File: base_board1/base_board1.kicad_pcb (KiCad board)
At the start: 4 copper layers, 99.4 x 100 mm, 161 parts, among them J1 DF40C-60DS-0.4V_51_, J2 DF40C-60DS-0.4V_51_, J3 Conn_01x30, J4 Conn_01x30, J5 Conn_01x30, J6 Conn_01x30

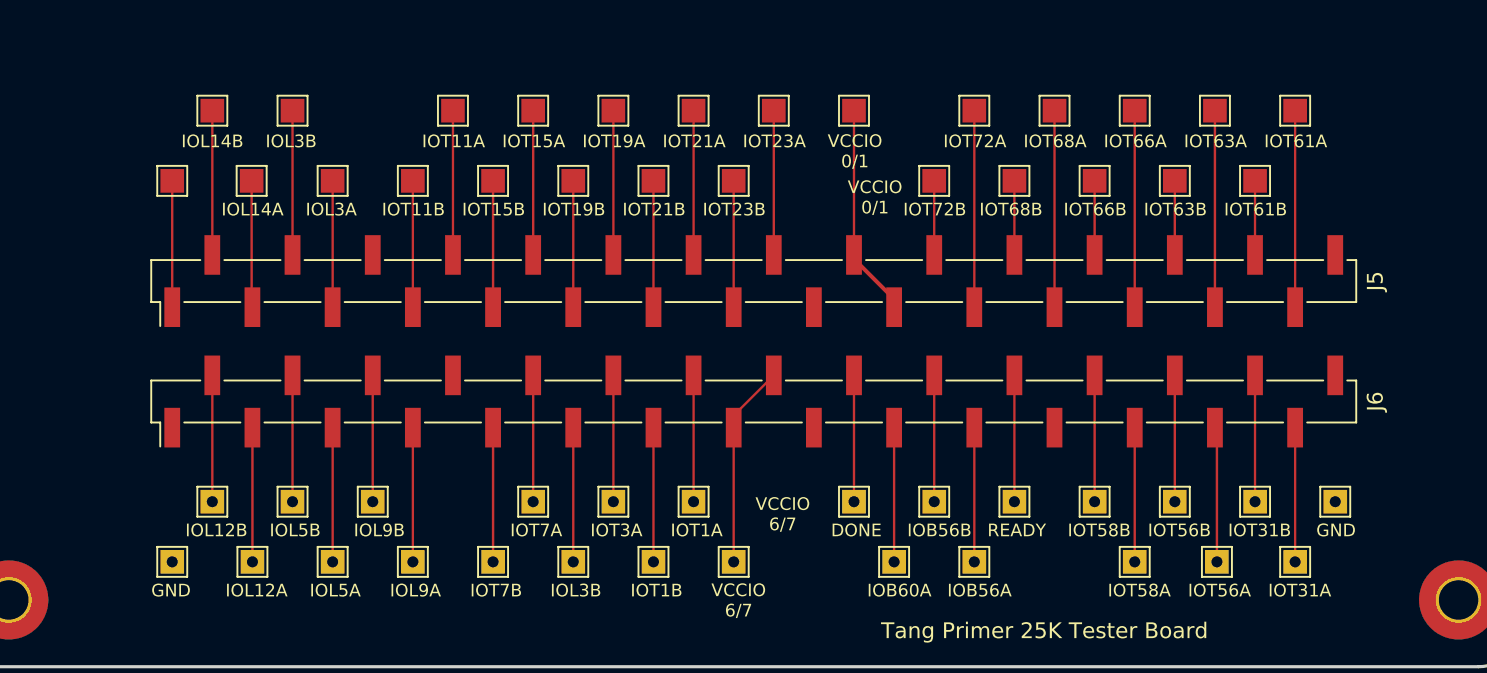
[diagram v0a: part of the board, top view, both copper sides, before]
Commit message: 1219
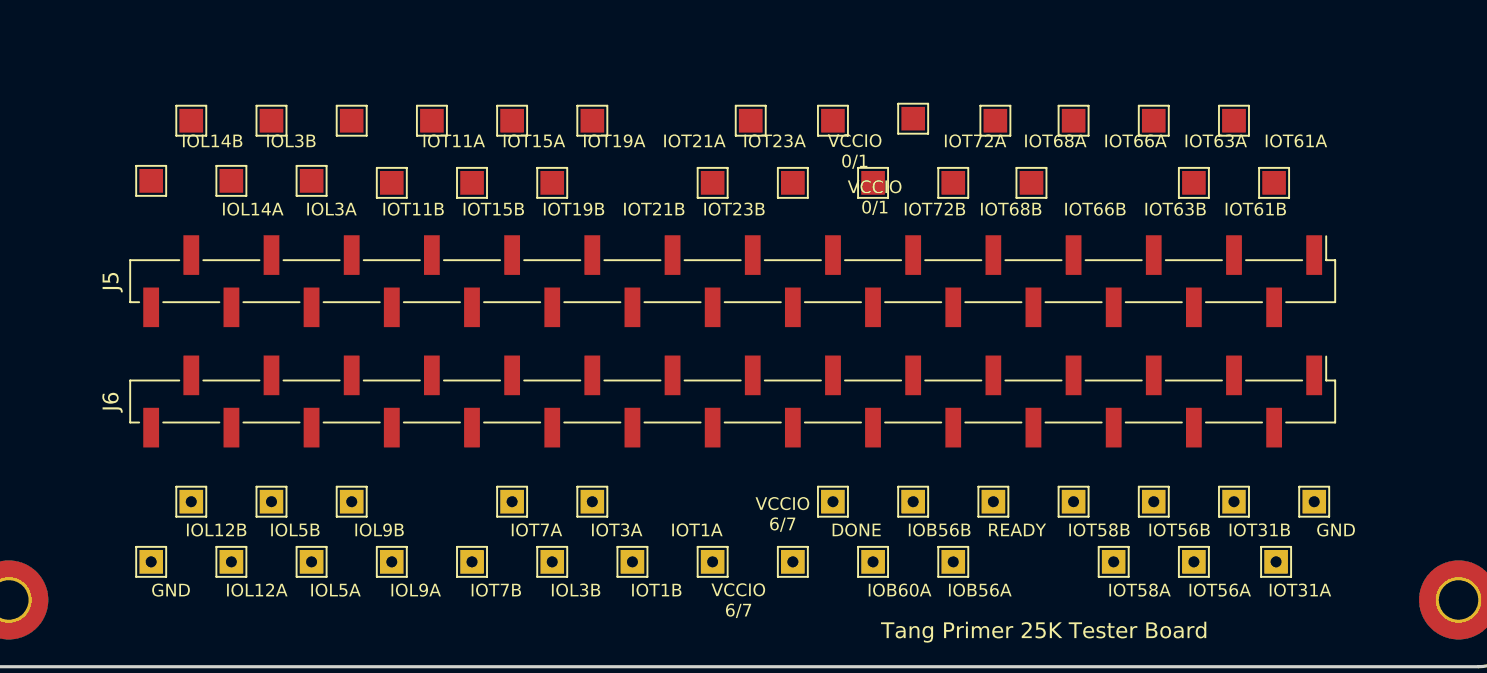
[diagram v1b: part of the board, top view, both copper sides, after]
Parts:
- moved TP69 70.0 mm to (137.3, 146.7)
- moved TP70 69.9 mm to (137.3, 122.6)
- moved TP123 67.5 mm to (206.0, 150.5)
- moved TP124 67.4 mm to (205.9, 126.5)
- moved TP71 64.9 mm to (139.8, 150.5)
- moved TP72 64.8 mm to (139.8, 126.4)
- moved TP122 62.3 mm to (203.3, 122.6)
- moved TP121 62.3 mm to (203.3, 146.7)
- moved TP73 60.0 mm to (142.4, 146.7)
- moved TP74 59.8 mm to (142.4, 122.6)
- moved TP120 57.3 mm to (200.8, 126.5)
- moved TP119 57.2 mm to (200.8, 150.5)
- moved TP75 54.8 mm to (144.9, 150.5)
- moved TP76 54.7 mm to (144.9, 126.4)
- moved TP117 52.1 mm to (198.2, 146.7)
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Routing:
- net /VCCIO0/1: track 13.8 -> 0.00 mm
- net /VCCIO6/7: track 12.9 -> 0.00 mm
- net /IOT72A: track 12.7 -> 0.00 mm
- net /IOT68A: track 12.7 -> 0.00 mm
- net /IOT66A: track 12.7 -> 0.00 mm
- net /IOT63A: track 12.7 -> 0.00 mm
- net /IOT61A: track 12.7 -> 0.00 mm
- net /IOT23A: track 9.39 -> 0.00 mm
- net /IOT21A: track 9.39 -> 0.00 mm
- net /IOT19A: track 9.39 -> 0.00 mm
- net /IOT15A: track 9.39 -> 0.00 mm
- net /IOT11A: track 9.39 -> 0.00 mm
- net /IOL3B: track 9.39 -> 0.00 mm
- net /IOL14B: track 9.39 -> 0.00 mm
- net /IOT56A: track 8.55 -> 0.00 mm
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
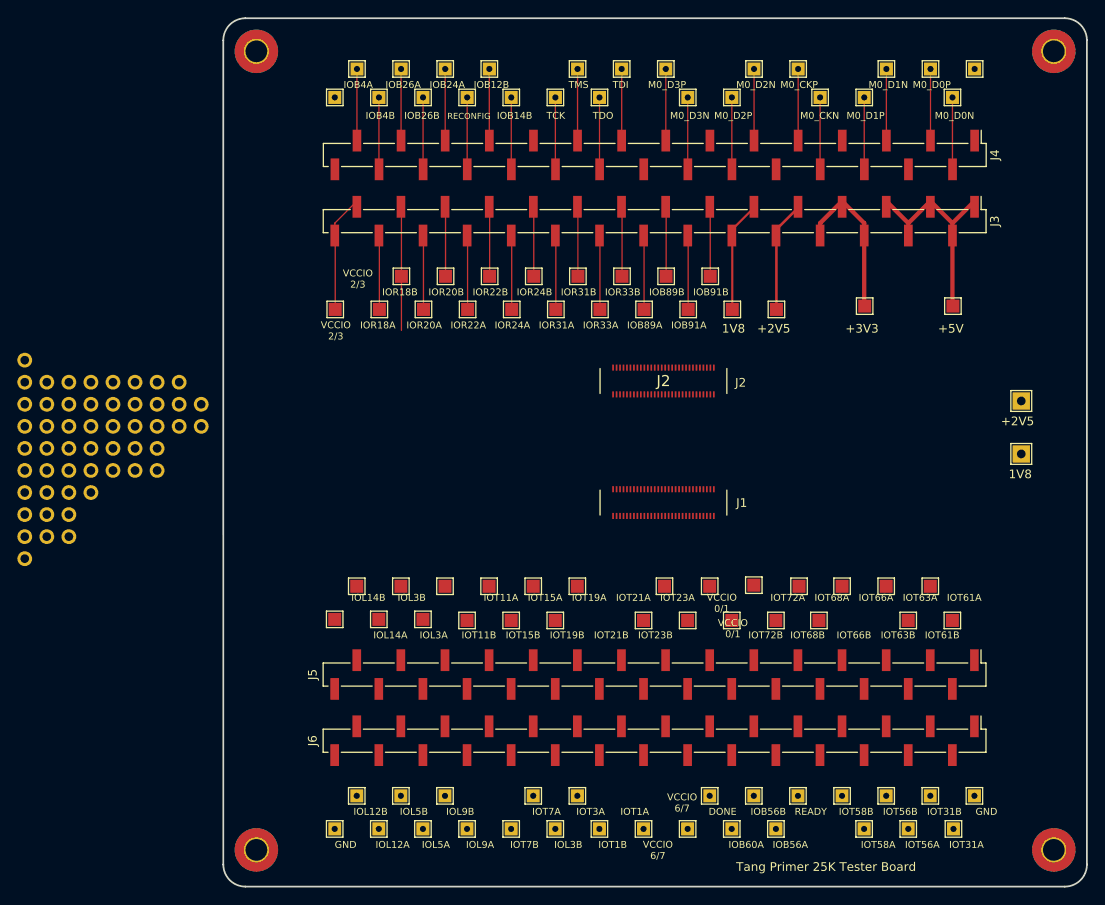
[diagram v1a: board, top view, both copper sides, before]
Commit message: 1220
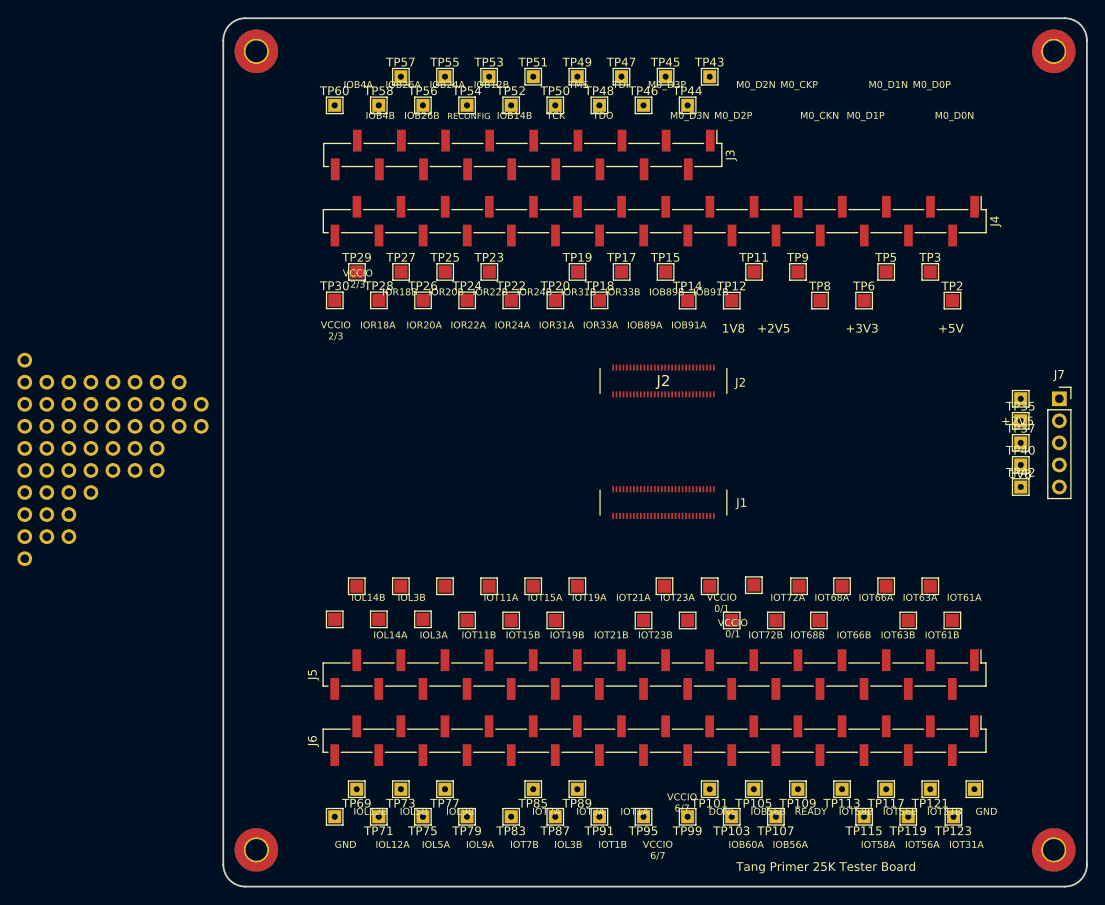
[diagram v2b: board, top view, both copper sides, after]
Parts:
- removed the REF** at (213.8, 101.2)
- removed the REF** at (213.8, 107.3)
- added J7: Conn_01x05, Connector_PinSocket_2.54mm:PinSocket_1x05_P2.54mm_Vertical, F.Cu at (218.2, 101.0)
- J3: value Conn_01x30 -> Conn_01x18; footprint Connector_PinHeader_2.54mm:PinHeader_1x30_P2.54mm_Vertical_SMD_Pin1Left -> Connector_PinHeader_2.54mm:PinHeader_1x18_P2.54mm_Vertical_SMD_Pin1Left
- TP11, TP12, TP14, TP15, TP17, TP18, TP19, TP2, TP20, TP22, TP23, TP24, TP25, TP26, TP27, TP28, TP29, TP3, TP30, TP5, TP6, TP8, TP9: footprint TestPoint:TestPoint_THTPad_1.5x1.5mm_Drill0.7mm -> TestPoint:TestPoint_Pad_1.5x1.5mm
- TP35, TP37, TP40, TP42, TP43, TP44, TP45, TP46, TP47, TP48, TP49, TP50, TP51, TP52, TP53, TP54, TP55, TP56, TP57, TP58, TP60: footprint TestPoint:TestPoint_Pad_1.5x1.5mm -> TestPoint:TestPoint_THTPad_1.5x1.5mm_Drill0.7mm
- moved TP42 39.0 mm to (213.7, 111.1)
- moved TP1 38.3 mm to (213.7, 101.0)
- moved TP40 33.3 mm to (213.7, 108.6)
- moved TP37 23.9 mm to (213.7, 106.0)
- moved TP44 23.5 mm to (175.4, 67.2)
- moved TP46 23.5 mm to (170.3, 67.2)
- moved TP48 23.5 mm to (165.2, 67.2)
- moved TP50 23.5 mm to (160.1, 67.2)
- moved TP52 23.5 mm to (155.1, 67.2)
- moved TP54 23.5 mm to (150.0, 67.2)
- moved TP56 23.5 mm to (144.9, 67.2)
- moved TP58 23.5 mm to (139.8, 67.2)
- moved TP60 23.5 mm to (134.7, 67.2)
- moved TP12 23.4 mm to (180.5, 89.7)
- moved TP14 23.4 mm to (175.4, 89.7)
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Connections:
- J1 pad 1: /GND -> GND
- J1 pad 15: /GND -> GND
- J1 pad 2: /GND -> GND
- J1 pad 27: /GND -> GND
- J1 pad 28: /GND -> GND
- J1 pad 45: /GND -> GND
- J1 pad 50: /GND -> GND
- J1 pad 59: /GND -> GND
- J1 pad 60: /GND -> GND
- J2 pad 1: /GND -> GND
- J2 pad 19: /GND -> GND
- J2 pad 29: /GND -> GND
- J2 pad 35: /GND -> GND
- J2 pad 41: /GND -> GND
- J2 pad 47: /GND -> GND
- J2 pad 53: /GND -> GND
- J2 pad 59: /GND -> GND
- J3 pad 1: +5V -> /IOB91B
- J3 pad 10: +2V5 -> /IOR24A
- J3 pad 11: /VDD_1V8 -> /IOR22B
- J3 pad 12: /VDD_1V8 -> /IOR22A
- J3 pad 13: /IOB91B -> /IOR20B
- J3 pad 14: /IOB91A -> /IOR20A
- J3 pad 15: /IOB89B -> /IOR18B
- J3 pad 16: /IOB89A -> /IOR18A
- J3 pad 17: /IOR33B -> /VCCIO2/3
- J3 pad 18: /IOR33A -> /VCCIO2/3
- J3 pad 2: +5V -> /IOB91A
- J3 pad 3: +5V -> /IOB89B
- J3 pad 4: +5V -> /IOB89A
- J3 pad 5: +5V -> /IOR33B
- J3 pad 6: +3V3 -> /IOR33A
- J3 pad 7: +3V3 -> /IOR31B
- J3 pad 8: +3V3 -> /IOR31A
- J3 pad 9: +2V5 -> /IOR24B
- J4 pad 1: /GND -> GND
- J4 pad 10: /GND -> GND
- J4 pad 13: /GND -> GND
- J4 pad 16: /GND -> GND
- J4 pad 21: /GND -> GND
- J4 pad 30: /GND -> GND
- J4 pad 4: /GND -> GND
- J4 pad 7: /GND -> GND
- J5 pad 1: /GND -> GND
- J5 pad 17: /GND -> GND
- J5 pad 30: /GND -> GND
- J5 pad 6: /GND -> GND
- J6 pad 1: /GND -> GND
- J6 pad 17: /GND -> GND
- J6 pad 23: /GND -> GND
- J6 pad 30: /GND -> GND
- J6 pad 8: /GND -> GND
- TP30 pad 1: /GND -> GND
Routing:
- net +5V: track 27.2 -> 0.00 mm
- net +3V3: track 20.8 -> 0.00 mm
- net /IOR18B: track 14.9 -> 0.00 mm
- net /VDD_1V8: track 13.5 -> 0.00 mm
- net /VCCIO2/3: track 13.5 -> 0.00 mm
- net +2V5: track 13.5 -> 0.00 mm
- net /IOR31A: track 9.18 -> 0.00 mm
- net /IOR24A: track 9.18 -> 0.00 mm
- net /IOR22A: track 9.18 -> 0.00 mm
- net /IOR20A: track 9.18 -> 0.00 mm
- net /IOB89A: track 9.18 -> 0.00 mm
- net /IOR33A: track 9.18 -> 0.00 mm
- net /IOR18A: track 9.18 -> 0.00 mm
- net /IOB91A: track 9.18 -> 0.00 mm
- net /IOR33B: track 8.68 -> 0.00 mm
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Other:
- copper layers 4 -> 2
